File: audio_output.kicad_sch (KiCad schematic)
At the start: 33 parts, among them J8 NCJ6FA-H-0, J9 NCJ6FA-H-0, U5 OPA1656ID, U6 THAT1646, U7 THAT1646

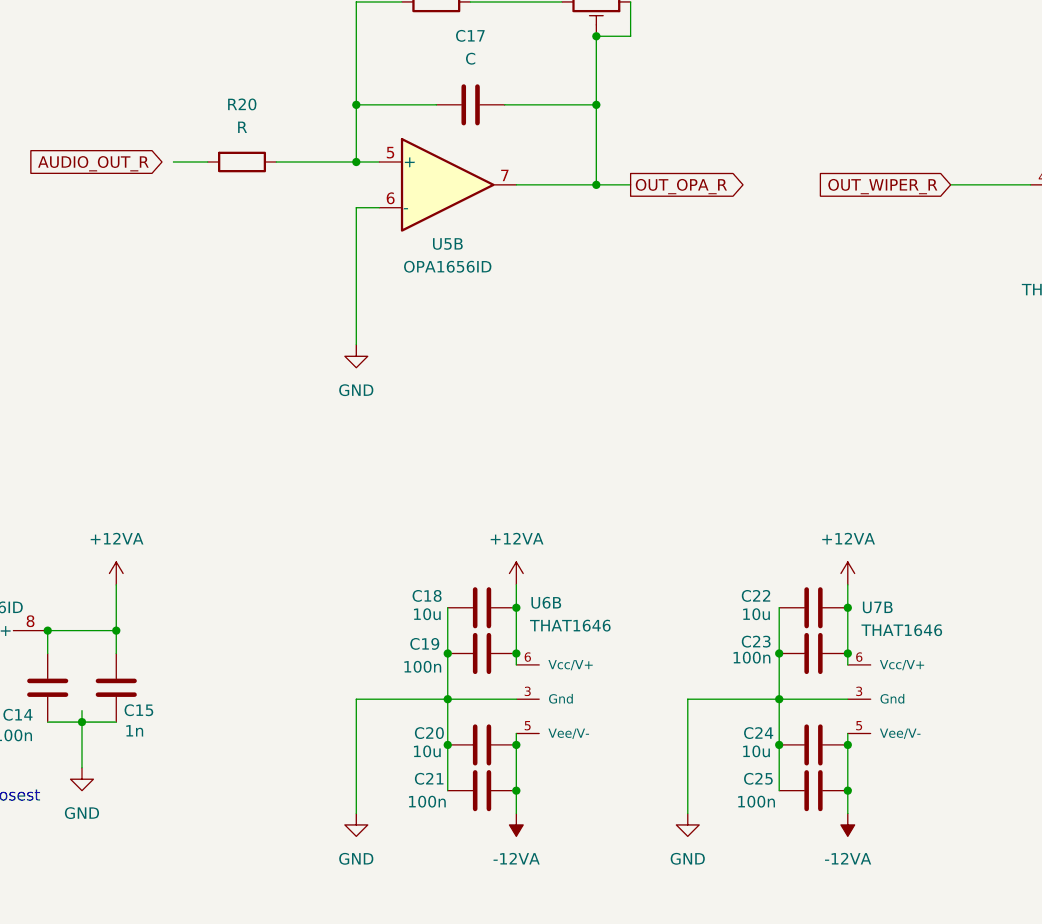
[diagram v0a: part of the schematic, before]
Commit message: TVS fix
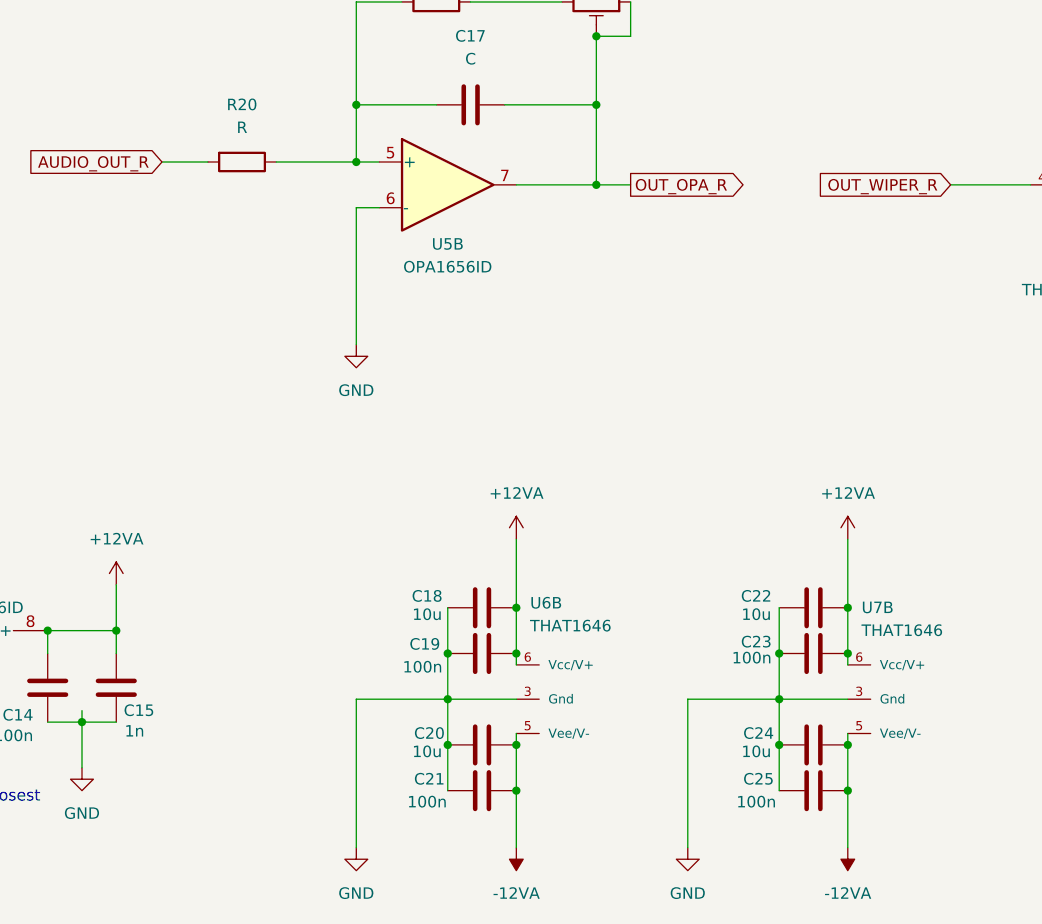
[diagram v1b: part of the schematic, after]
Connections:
- net AUDIO_OUT_R: now also R20.2
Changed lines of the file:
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@@
 	(wire
 		(pts
-			(xy 60.96 119.38) (xy 64.77 119.38)
-		)
-		(stroke
-			(width 0)
-			(type default)
-		)
-	)
-	(wire
-		(pts
-			(xy 99.06 166.37) (xy 99.06 168.91)
+			(xy 99.06 161.29) (xy 99.06 168.91)
 		)
 		(stroke
@@
 	(wire
 		(pts
-			(xy 81.28 191.77) (xy 81.28 179.07)
+			(xy 81.28 195.58) (xy 81.28 179.07)
 		)
 		(stroke
@@
 	(wire
 		(pts
-			(xy 135.89 166.37) (xy 135.89 168.91)
+			(xy 135.89 161.29) (xy 135.89 168.91)
 		)
 		(stroke
@@
 	(wire
 		(pts
-			(xy 99.06 189.23) (xy 99.06 191.77)
+			(xy 99.06 189.23) (xy 99.06 195.58)
 		)
 		(stroke
@@
 	(wire
 		(pts
-			(xy 118.11 191.77) (xy 118.11 179.07)
+			(xy 118.11 195.58) (xy 118.11 179.07)
 		)
 		(stroke
@@
 	(wire
 		(pts
-			(xy 135.89 189.23) (xy 135.89 191.77)
+			(xy 135.89 189.23) (xy 135.89 195.58)
 		)
 		(stroke
@@
 	(wire
 		(pts
+			(xy 59.69 119.38) (xy 64.77 119.38)
+		)
+		(stroke
+			(width 0)
+			(type default)
+		)
+	)
+	(wire
+		(pts
 			(xy 147.32 55.88) (xy 156.21 55.88)
 		)
@@
 	(symbol
 		(lib_id "power:+12VA")
-		(at 99.06 166.37 0)
+		(at 99.06 161.29 0)
 		(unit 1)
 		(exclude_from_sim no)
@@
 		(fields_autoplaced yes)
 		(property "Reference" "#PWR036"
-			(at 99.06 170.18 0)
+			(at 99.06 165.1 0)
 			(effects
 				(font
@@
 		)
 		(property "Value" "+12VA"
-			(at 99.06 161.29 0)
+			(at 99.06 156.21 0)
 			(effects
 				(font
@@
 		)
 		(property "Footprint" ""
-			(at 99.06 166.37 0)
+			(at 99.06 161.29 0)
 			(effects
 				(font
@@
 		)
 		(property "Datasheet" ""
-			(at 99.06 166.37 0)
+			(at 99.06 161.29 0)
 			(effects
 				(font
@@
 		)
 		(property "Description" "Power symbol creates a global label with name \"+12VA\""
-			(at 99.06 166.37 0)
+			(at 99.06 161.29 0)
 			(effects
 				(font
@@
 	(symbol
 		(lib_id "power:-12VA")
-		(at 99.06 191.77 180)
+		(at 99.06 195.58 180)
 		(unit 1)
 		(exclude_from_sim no)
@@
 		(fields_autoplaced yes)
 		(property "Reference" "#PWR037"
-			(at 99.06 187.96 0)
+			(at 99.06 191.77 0)
 			(effects
 				(font
@@
 		)
 		(property "Value" "-12VA"
-			(at 99.06 196.85 0)
+			(at 99.06 200.66 0)
 			(effects
 				(font
@@
 		)
 		(property "Footprint" ""
-			(at 99.06 191.77 0)
+			(at 99.06 195.58 0)
 			(effects
 				(font
@@
 		)
 		(property "Datasheet" ""
-			(at 99.06 191.77 0)
+			(at 99.06 195.58 0)
 			(effects
 				(font
@@
 		)
 		(property "Description" "Power symbol creates a global label with name \"-12VA\""
-			(at 99.06 191.77 0)
+			(at 99.06 195.58 0)
 			(effects
 				(font
@@
 	(symbol
 		(lib_id "power:-12VA")
-		(at 135.89 191.77 180)
+		(at 135.89 195.58 180)
 		(unit 1)
 		(exclude_from_sim no)
@@
 		(fields_autoplaced yes)
 		(property "Reference" "#PWR040"
-			(at 135.89 187.96 0)
+			(at 135.89 191.77 0)
 			(effects
 				(font
@@
 		)
 		(property "Value" "-12VA"
-			(at 135.89 196.85 0)
+			(at 135.89 200.66 0)
 			(effects
 				(font
@@
 		)
 		(property "Footprint" ""
-			(at 135.89 191.77 0)
+			(at 135.89 195.58 0)
 			(effects
 				(font
@@
 		)
 		(property "Datasheet" ""
-			(at 135.89 191.77 0)
+			(at 135.89 195.58 0)
 			(effects
 				(font
@@
 		)
 		(property "Description" "Power symbol creates a global label with name \"-12VA\""
-			(at 135.89 191.77 0)
+			(at 135.89 195.58 0)
 			(effects
 				(font
@@
 	(symbol
 		(lib_id "power:GND")
-		(at 81.28 191.77 0)
+		(at 81.28 195.58 0)
 		(unit 1)
 		(exclude_from_sim no)
@@
 		(fields_autoplaced yes)
 		(property "Reference" "#PWR035"
-			(at 81.28 198.12 0)
+			(at 81.28 201.93 0)
 			(effects
 				(font
@@
 		)
 		(property "Value" "GND"
-			(at 81.28 196.85 0)
+			(at 81.28 200.66 0)
 			(effects
 				(font
@@
 		)
 		(property "Footprint" ""
-			(at 81.28 191.77 0)
+			(at 81.28 195.58 0)
 			(effects
 				(font
@@
 		)
 		(property "Datasheet" ""
-			(at 81.28 191.77 0)
+			(at 81.28 195.58 0)
 			(effects
 				(font
@@
 		)
 		(property "Description" "Power symbol creates a global label with name \"GND\" , ground"
-			(at 81.28 191.77 0)
+			(at 81.28 195.58 0)
 			(effects
 				(font
@@
 	(symbol
 		(lib_id "power:+12VA")
-		(at 135.89 166.37 0)
+		(at 135.89 161.29 0)
 		(unit 1)
 		(exclude_from_sim no)
@@
 		(fields_autoplaced yes)
 		(property "Reference" "#PWR039"
-			(at 135.89 170.18 0)
+			(at 135.89 165.1 0)
 			(effects
 				(font
@@
 		)
 		(property "Value" "+12VA"
-			(at 135.89 161.29 0)
+			(at 135.89 156.21 0)
 			(effects
 				(font
@@
 		)
 		(property "Footprint" ""
-			(at 135.89 166.37 0)
+			(at 135.89 161.29 0)
 			(effects
 				(font
@@
 		)
 		(property "Datasheet" ""
-			(at 135.89 166.37 0)
+			(at 135.89 161.29 0)
 			(effects
 				(font
@@
 		)
 		(property "Description" "Power symbol creates a global label with name \"+12VA\""
-			(at 135.89 166.37 0)
+			(at 135.89 161.29 0)
 			(effects
 				(font
@@
 	(symbol
 		(lib_id "power:GND")
-		(at 118.11 191.77 0)
+		(at 118.11 195.58 0)
 		(unit 1)
 		(exclude_from_sim no)
@@
 		(fields_autoplaced yes)
 		(property "Reference" "#PWR038"
-			(at 118.11 198.12 0)
+			(at 118.11 201.93 0)
 			(effects
 				(font
@@
 		)
 		(property "Value" "GND"
-			(at 118.11 196.85 0)
+			(at 118.11 200.66 0)
 			(effects
 				(font
@@
 		)
 		(property "Footprint" ""
-			(at 118.11 191.77 0)
+			(at 118.11 195.58 0)
 			(effects
 				(font
@@
 		)
 		(property "Datasheet" ""
-			(at 118.11 191.77 0)
+			(at 118.11 195.58 0)
 			(effects
 				(font
@@
 		)
 		(property "Description" "Power symbol creates a global label with name \"GND\" , ground"
-			(at 118.11 191.77 0)
+			(at 118.11 195.58 0)
 			(effects
 				(font

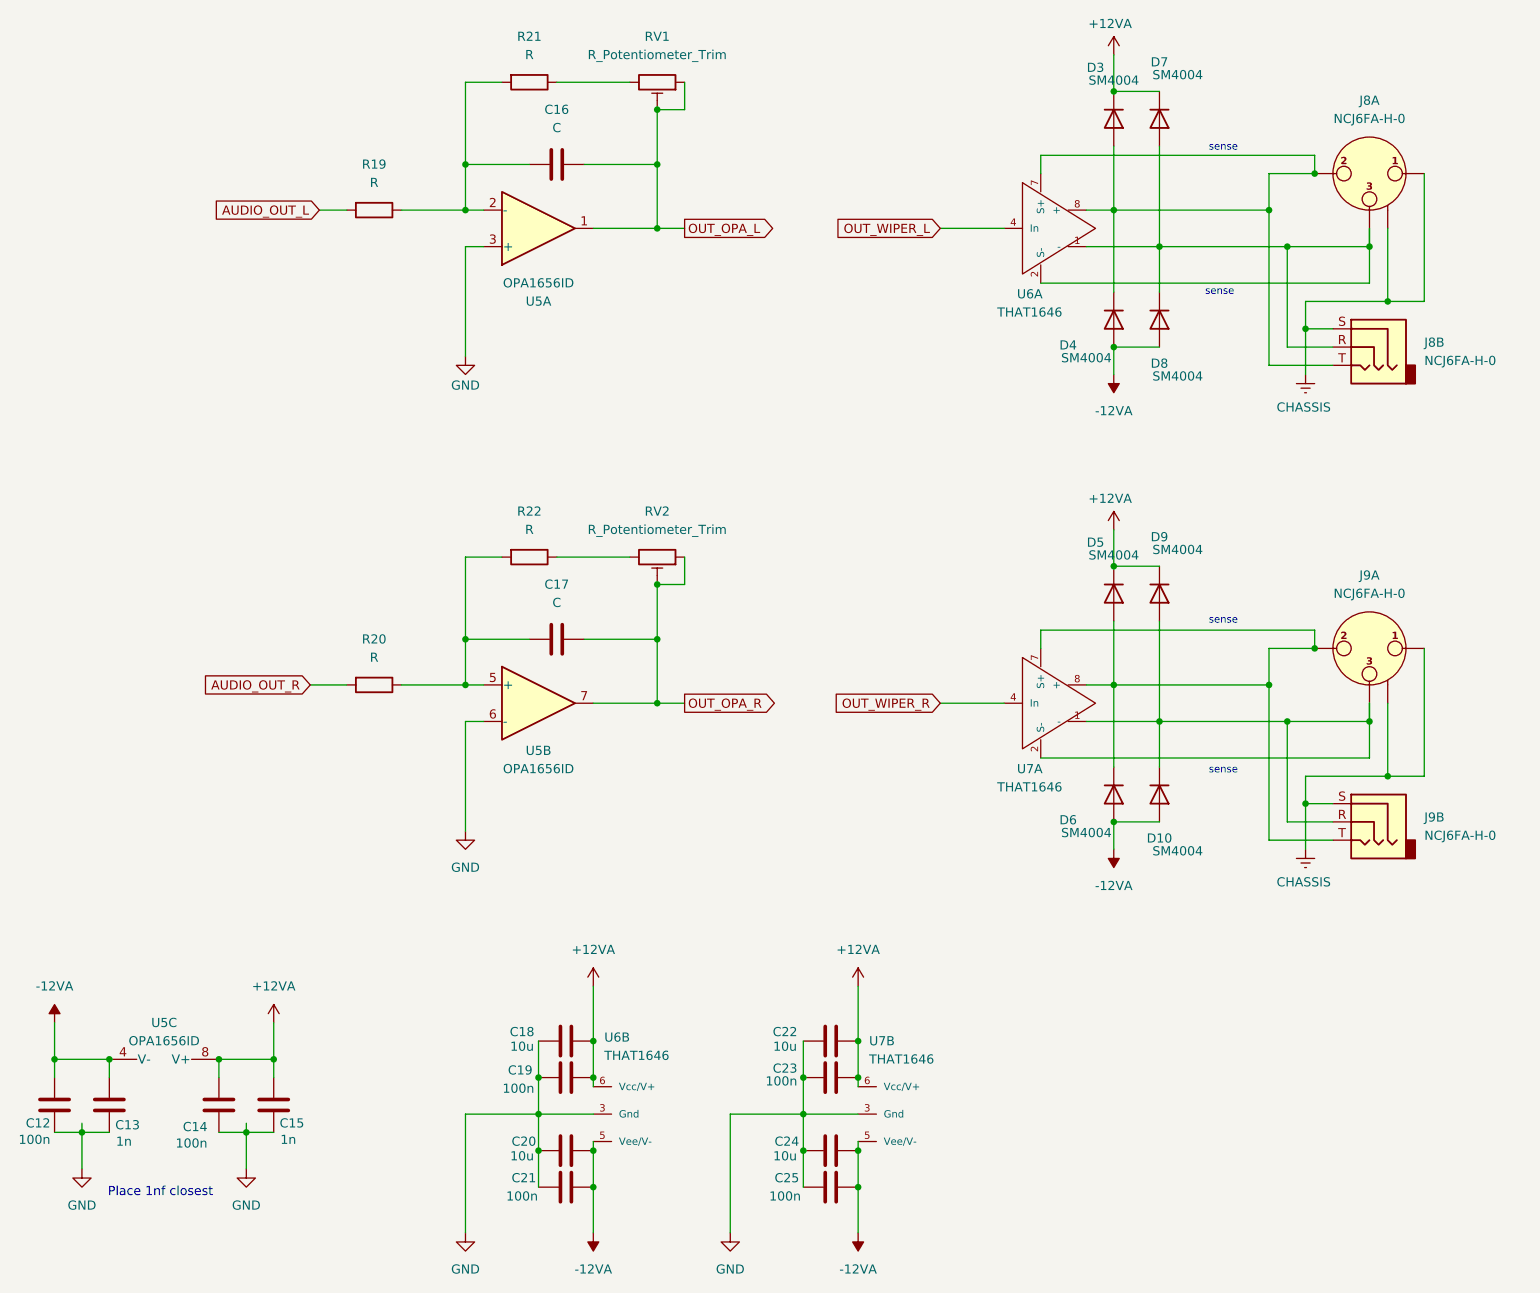
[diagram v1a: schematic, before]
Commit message: working on output
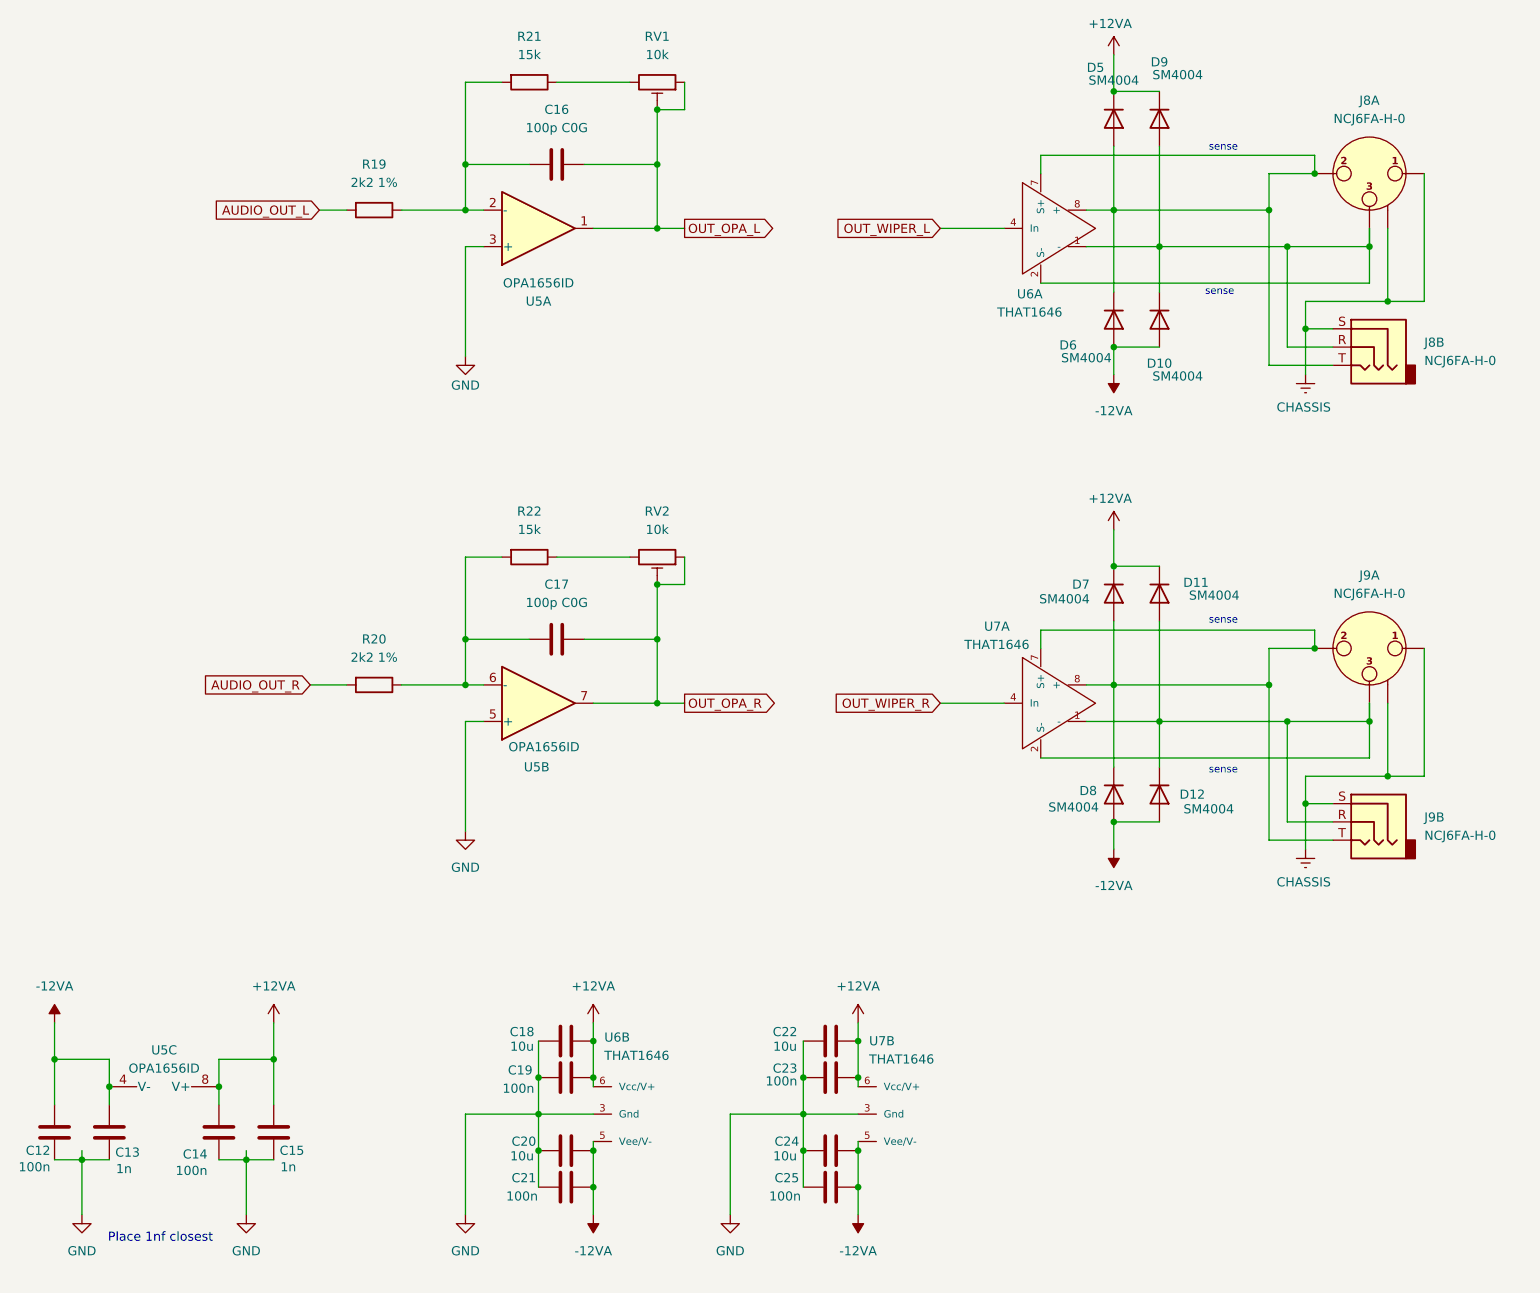
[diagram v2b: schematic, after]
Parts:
- C16, C17: value C -> 100p C0G
- R19, R20: value R -> 2k2 1%
- R21, R22: value R -> 15k
- RV1, RV2: value R_Potentiometer_Trim -> 10k
- renumbered D8 to D10, D9 to D11, D10 to D12, D3 to D5, D4 to D6, D5 to D7, D6 to D8, D7 to D9
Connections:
- net GND: now also U5.5 (+); no longer U5.6 (-)
- net at C17.1, R20.1, R22.2: now also U5.6 (-); no longer U5.5 (+)
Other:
- moved on the sheet: C12, C13, C14, C15, U5C
